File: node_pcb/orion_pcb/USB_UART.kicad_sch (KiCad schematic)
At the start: 19 parts, among them J301 USB_B_Micro, Q301 PJA3405, U301 SRV05-4A, U302 NCV8161ASN330T1G, U303 CP2102N-A02-GQFN24

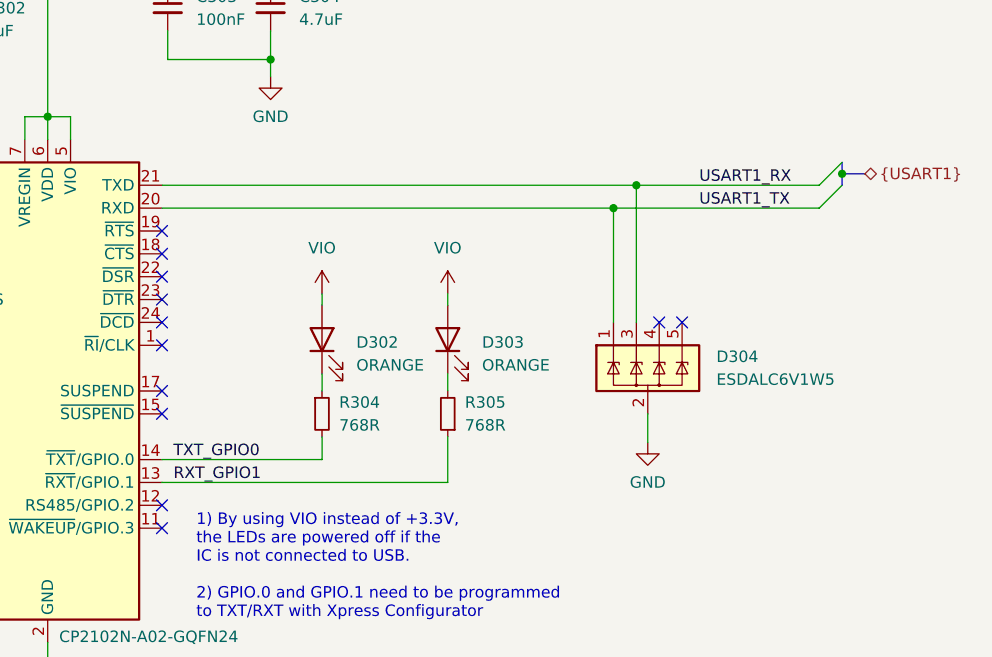
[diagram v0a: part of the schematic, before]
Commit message: Partial layout with max3232. To change to max3225
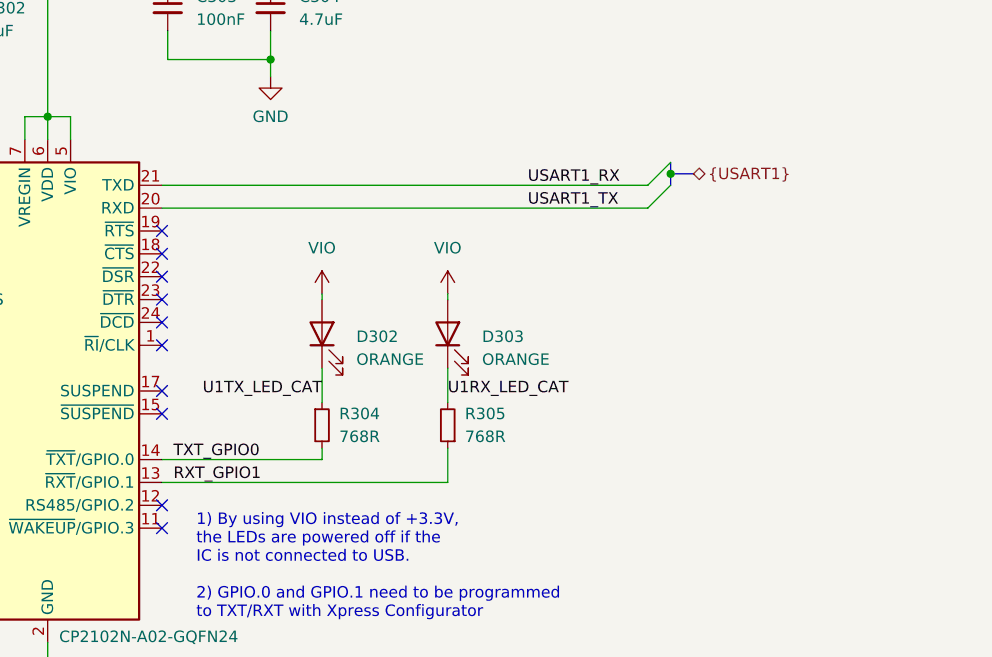
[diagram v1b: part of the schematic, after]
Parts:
- removed D304: ESDALC6V1W5, Package_TO_SOT_SMD:SOT-23-5, symbol 0_power_protection:ESDALC6V1W5
- C301, C302, C303, C304: footprint (none) -> Capacitor_SMD:C_0603_1608Metric
- R301, R302, R303, R304, R305: footprint (none) -> Resistor_SMD:R_0603_1608Metric
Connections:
- net U1TX_LED_CAT: now reaches D302.1 (K), R304.1
- net U1RX_LED_CAT: now reaches D303.1 (K), R305.2
- no-connect marks 15 -> 13
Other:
- moved on the sheet: D302, D303, R304, R305

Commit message: updated paths
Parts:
- J301: footprint Connector_USB:USB_Micro-B_Molex-105017-0001 -> 0_connectors:USB_Micro-B_Molex-105017-0001
- U302: Digikey ref (none) -> NCV8161ASN330T1GOSCT-ND; Manufacturer ref  (none) -> NCV8161ASN330T1G
- U303: Digikey ref (none) -> 1175-1628-ND; Manufacturer ref (none) -> 3220-10-0200-00
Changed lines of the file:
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@@
     (property "Reference" "J301" (id 0) (at 29.21 57.785 0))
     (property "Value" "USB_B_Micro" (id 1) (at 29.21 60.325 0))
-    (property "Footprint" "Connector_USB:USB_Micro-B_Molex-105017-0001" (id 2) (at 33.02 72.39 0)
+    (property "Footprint" "0_connectors:USB_Micro-B_Molex-105017-0001" (id 2) (at 33.02 72.39 0)
       (effects (font (size 1.27 1.27)) hide)
     )
@@
     )
     (property "Datasheet" "https://www.silabs.com/documents/public/data-sheets/cp2102n-datasheet.pdf" (id 3) (at 171.45 112.395 0)
+      (effects (font (size 1.27 1.27)) hide)
+    )
+    (property "Manufacturer ref" "3220-10-0200-00" (id 4) (at 171.45 113.665 0)
+      (effects (font (size 1.27 1.27)) hide)
+    )
+    (property "Digikey ref" "1175-1628-ND" (id 5) (at 171.45 113.665 0)
       (effects (font (size 1.27 1.27)) hide)
     )
@@
       (effects (font (size 1.27 1.27)) hide)
     )
+    (property "Manufacturer ref " "NCV8161ASN330T1G" (id 4) (at 150.495 68.58 0)
+      (effects (font (size 1.27 1.27)) hide)
+    )
+    (property "Digikey ref" "NCV8161ASN330T1GOSCT-ND" (id 5) (at 150.495 68.58 0)
+      (effects (font (size 1.27 1.27)) hide)
+    )

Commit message: ädded BOM
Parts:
- U302: Manufacturer ref (none) -> NCV8161ASN330T1G; Manufacturer ref  NCV8161ASN330T1G -> (none)
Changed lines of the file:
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@@
       (effects (font (size 1.27 1.27)) hide)
     )
-    (property "Manufacturer ref " "NCV8161ASN330T1G" (id 4) (at 150.495 68.58 0)
+    (property "Manufacturer ref" "NCV8161ASN330T1G" (id 4) (at 150.495 68.58 0)
       (effects (font (size 1.27 1.27)) hide)
     )
